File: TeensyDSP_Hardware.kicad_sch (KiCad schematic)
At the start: 14 parts, among them J1 AudioJack2, U1 DM-OLED096-636, U2 TL072, U5 Teensy4.0

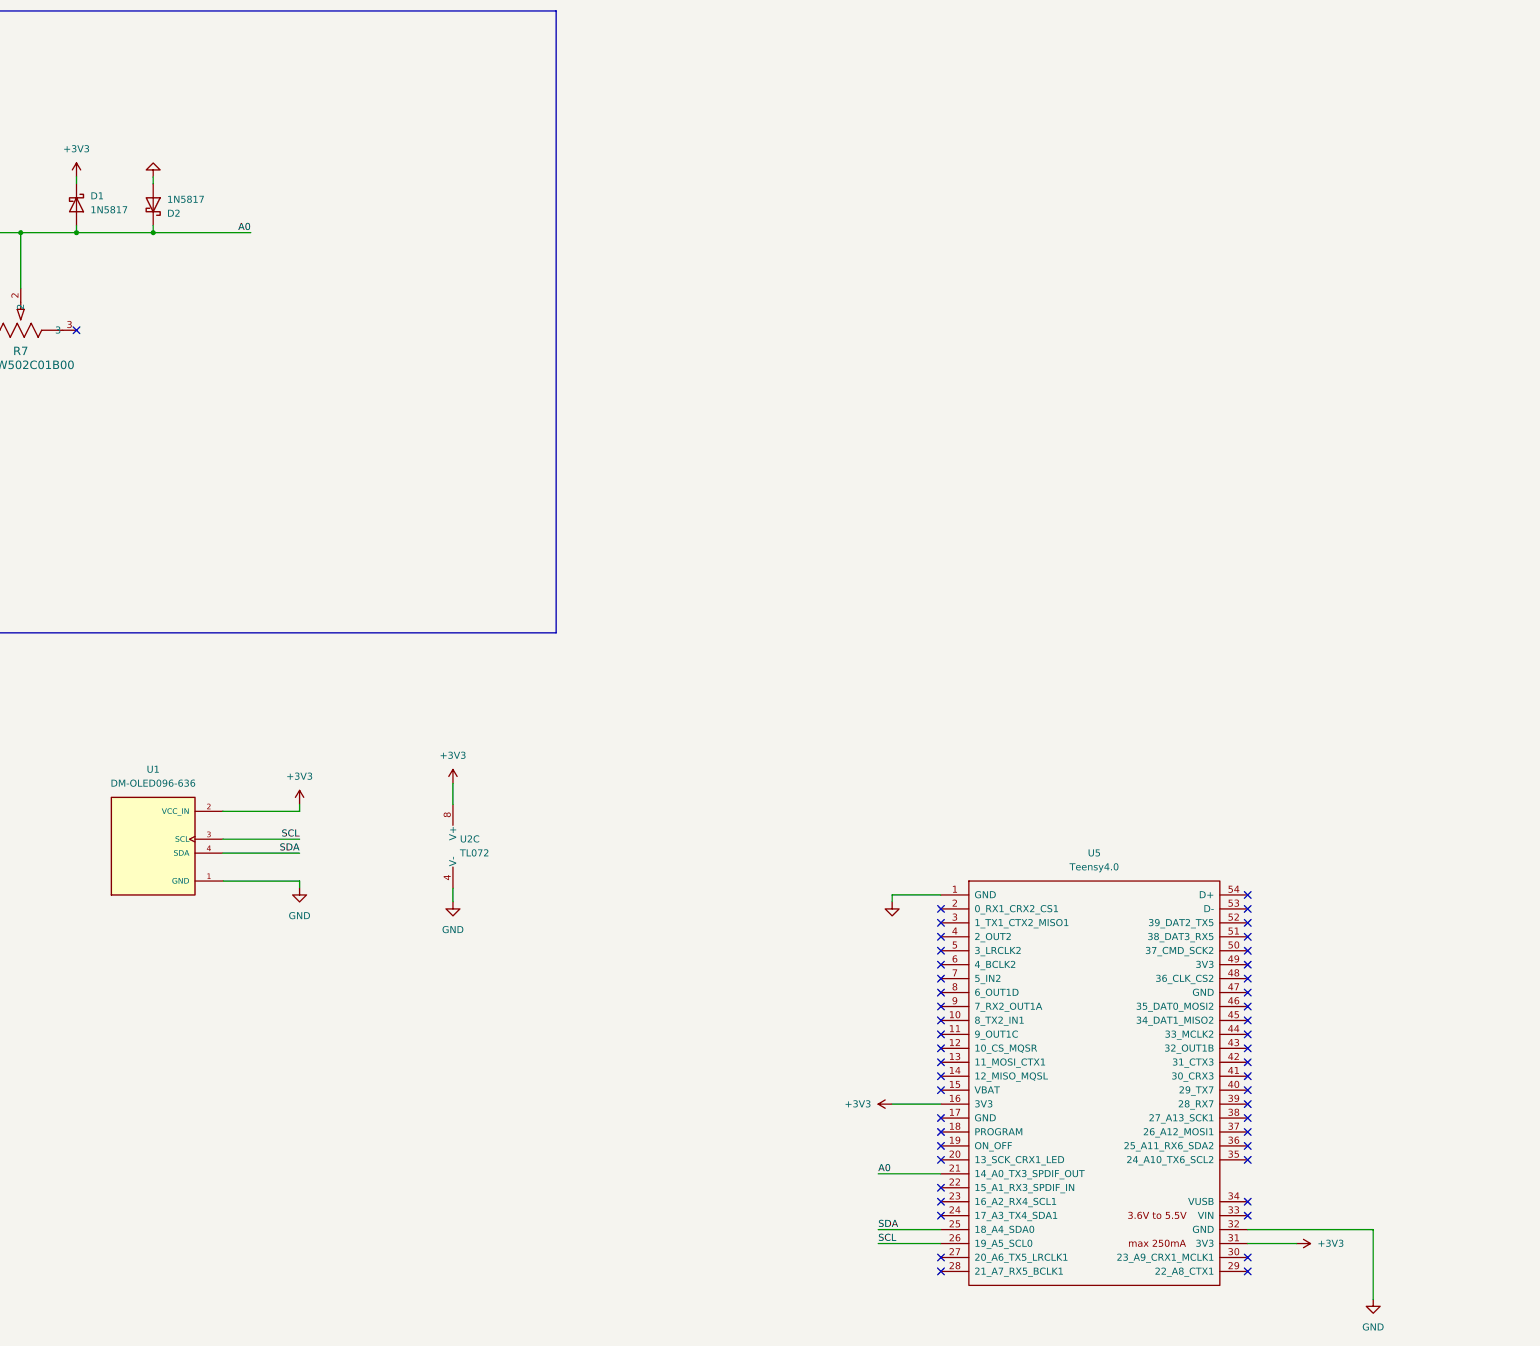
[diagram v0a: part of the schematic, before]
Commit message: move toward guitar tuner
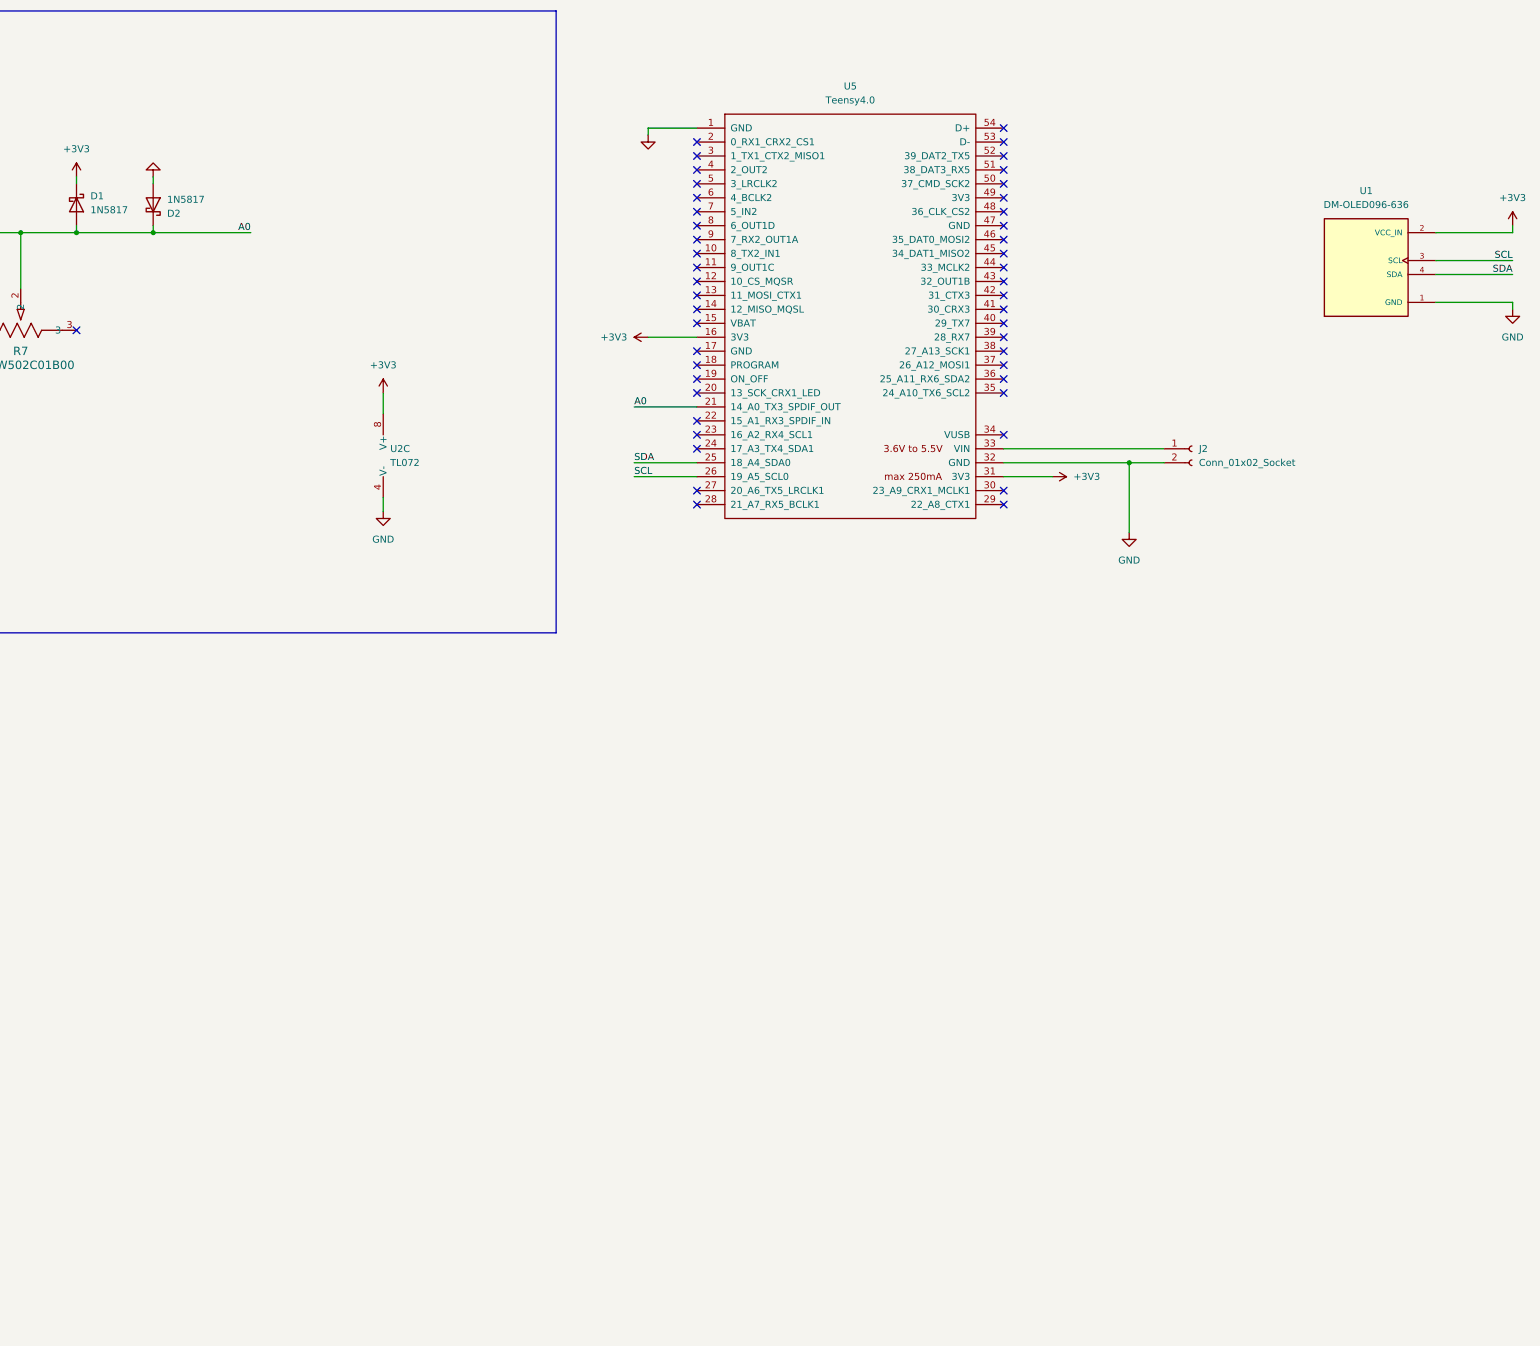
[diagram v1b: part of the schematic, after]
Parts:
- added J2: Conn_01x02_Socket, Connector_JST:JST_EH_B2B-EH-A_1x02_P2.50mm_Vertical, symbol Connector:Conn_01x02_Socket
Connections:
- net GND: now also J2.2 (Pin_2)
- net at U5.33 (VIN): now also J2.1 (Pin_1)
- no-connect marks 51 -> 50
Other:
- moved on the sheet: U1, U2C, U5
